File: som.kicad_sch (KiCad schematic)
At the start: 30 parts, among them J14 Conn_01x04, M1 jetson-orin-nx/nano-module, Q1 PJE138K, U4 NTS0102GT

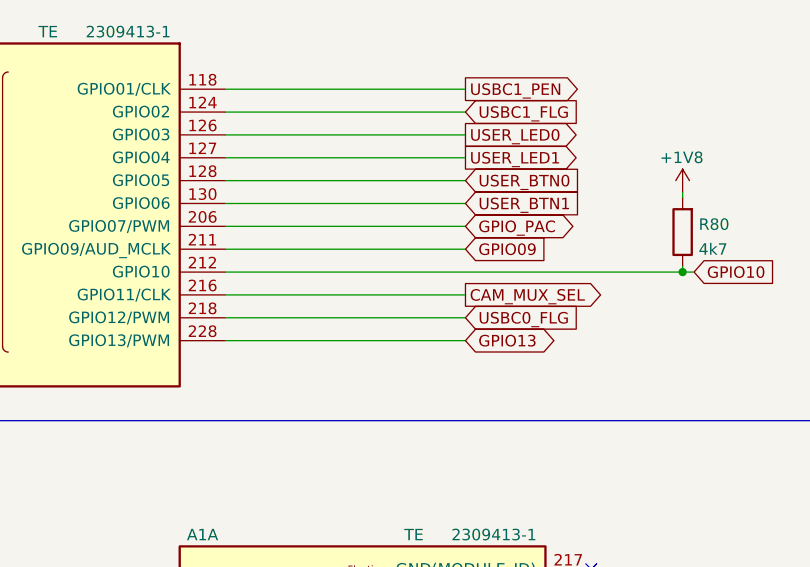
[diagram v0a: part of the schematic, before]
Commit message: Small changes
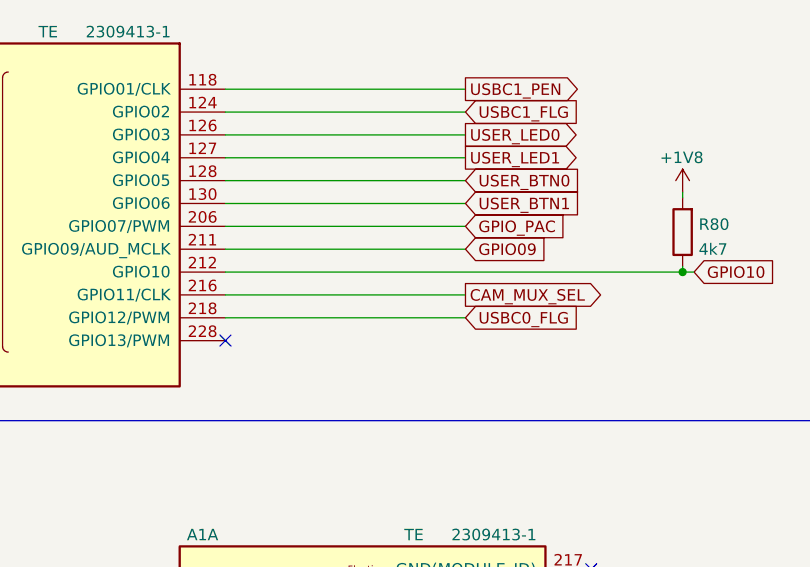
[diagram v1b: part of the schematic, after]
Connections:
- net GPIO13: no longer names the net of A1.228 (GPIO13/PWM)
- no-connect marks 64 -> 65
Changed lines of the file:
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@@
   (no_connect (at 367.03 111.76))
   (no_connect (at 189.23 134.62))
+  (no_connect (at 68.58 58.42))
   (no_connect (at 367.03 129.54))
   (no_connect (at 189.23 236.22))
@@
     (stroke (width 0) (type default))
   )
-  (wire (pts (xy 68.58 58.42) (xy 95.25 58.42))
-    (stroke (width 0) (type default))
-  )
   (wire (pts (xy 367.03 66.04) (xy 377.19 66.04))
     (stroke (width 0) (type default))
@@
     )
   )
-  (global_label "GPIO_PAC" (shape bidirectional) (at 95.25 45.72 0)
+  (global_label "GPIO_PAC" (shape input) (at 95.25 45.72 0)
     (effects (font (size 1.27 1.27)) (justify left))
     (property "Intersheetrefs" "${INTERSHEET_REFS}" (at 109.855 45.72 0)
@@
     )
   )
-  (global_label "GPIO13" (shape bidirectional) (at 95.25 58.42 0)
-    (effects (font (size 1.27 1.27)) (justify left))
-    (property "Intersheetrefs" "${INTERSHEET_REFS}" (at 109.855 58.42 0)
-      (effects (font (size 1.27 1.27)) (justify left))
-    )
-  )

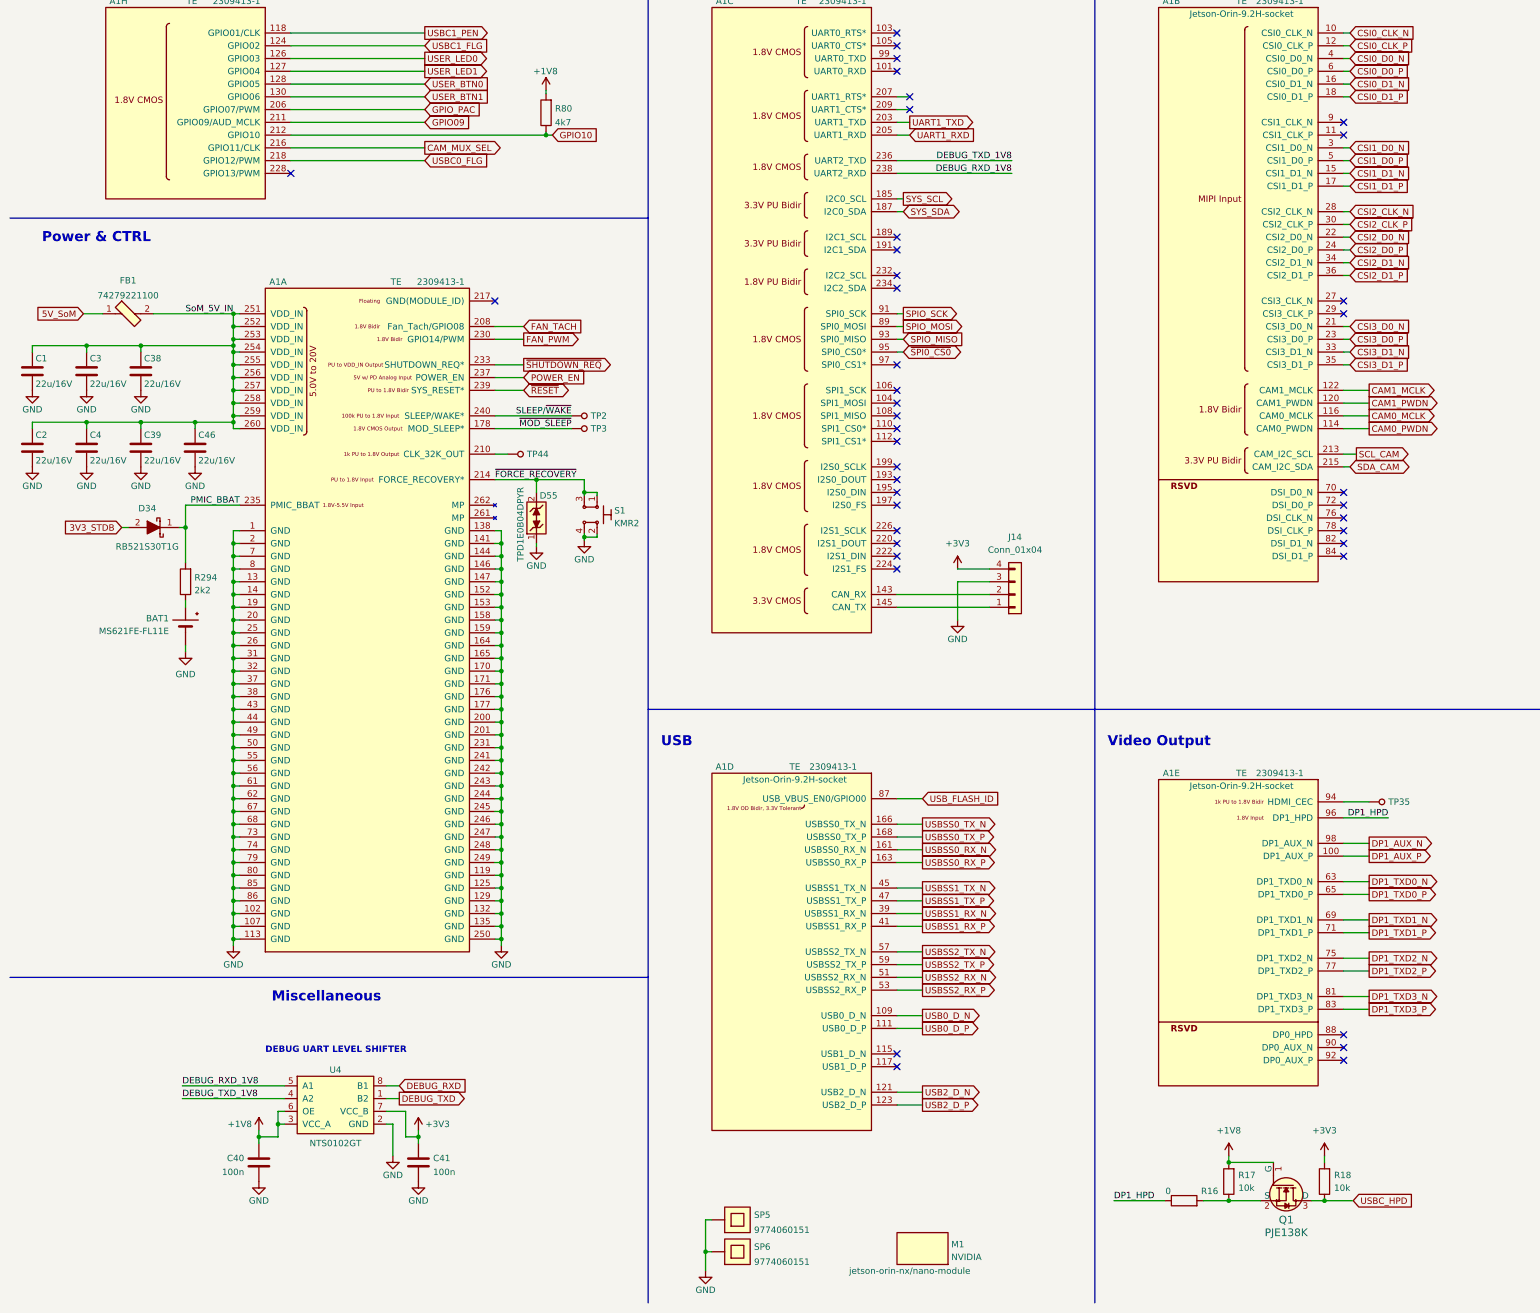
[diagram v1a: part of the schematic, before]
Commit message: Schematic Done
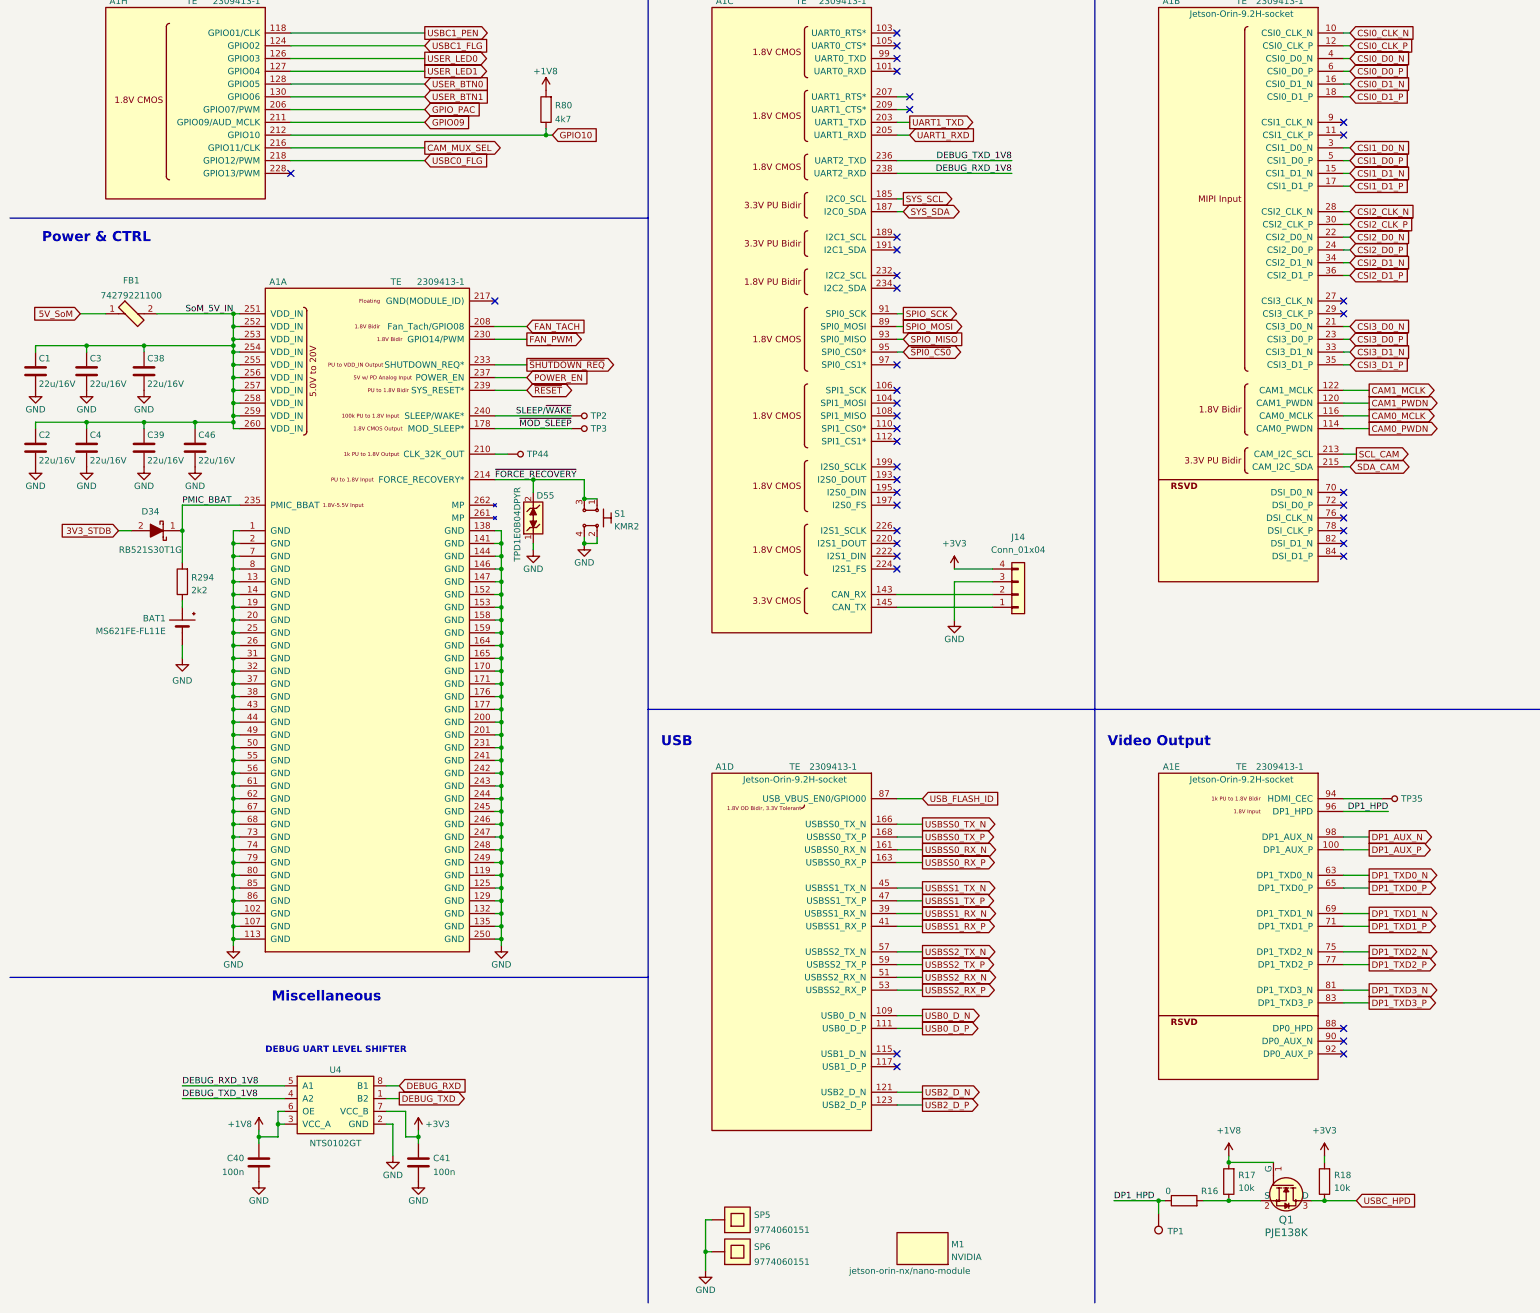
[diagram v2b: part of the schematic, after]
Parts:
- added TP1: TestPoint, symbol Connector:TestPoint
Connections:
- net DP1_HPD: now also TP1.1
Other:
- moved on the sheet: A1E, BAT1, C1, C2, C38, C39, D34, D55, FB1, J14, R294, R80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
